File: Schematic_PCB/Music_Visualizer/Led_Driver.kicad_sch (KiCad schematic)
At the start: 92 parts, among them U10 LM3915N-1, U11 LM3915N-1, U12 LM3915N-1, U13 LM3915N-1, U14 LM3915N-1, U15 LM3915N-1, U16 LM3915N-1, U17 NCP161ASN350T1G

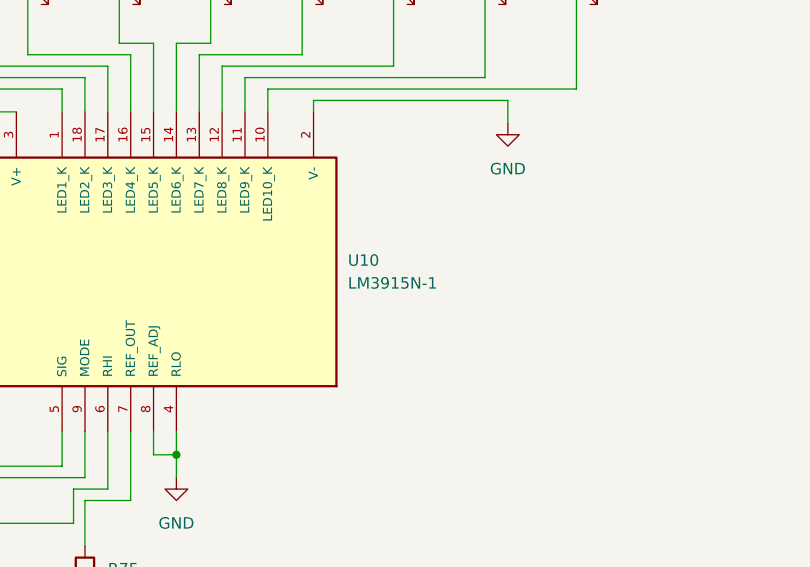
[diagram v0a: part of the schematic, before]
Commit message: Delete unused LED step and fooprint files in the Project library
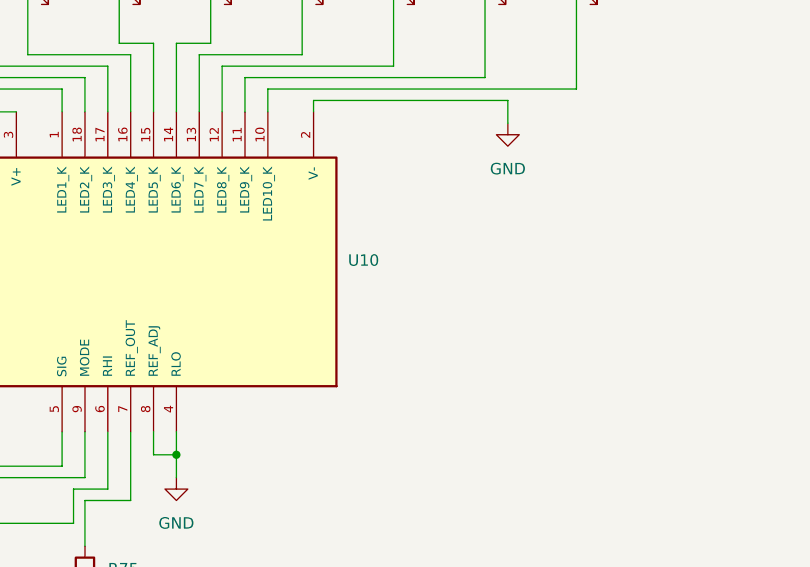
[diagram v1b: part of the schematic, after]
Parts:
- U10: value LM3915N-1 -> (none); footprint Package_DIP:DIP-18_W7.62mm_Socket -> (none)
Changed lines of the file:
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@@
       (effects (font (size 1.27 1.27)) (justify right))
     )
-    (property "Value" "LM3915N-1" (id 1) (at 118.11 90.1699 90)
+    (property "Value" "" (id 1) (at 118.11 90.1699 90)
       (effects (font (size 1.27 1.27)) (justify right))
     )
-    (property "Footprint" "Package_DIP:DIP-18_W7.62mm_Socket" (id 2) (at 96.52 88.9 0)
+    (property "Footprint" "" (id 2) (at 96.52 88.9 0)
       (effects (font (size 1.27 1.27)) (justify left bottom) hide)
     )

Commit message: Rearraged Power circuitry schematic and made the paper size custom: 180W x 250H
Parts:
- RV1: value (none) -> 10k_LED_Brightness_Pot; footprint (none) -> PTV09A_Pot_Vertical:PTV09
- U10: value (none) -> LM3915N-1; footprint (none) -> Package_DIP:DIP-18_W7.62mm_Socket
- U18: value (none) -> NCS333ASQ3T2G; footprint (none) -> Package_TO_SOT_SMD:SOT-353_SC-70-5
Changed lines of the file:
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@@
       (effects (font (size 1.27 1.27)) (justify right))
     )
-    (property "Value" "" (id 1) (at 355.6 212.0899 0)
-      (effects (font (size 1.27 1.27)) (justify right))
-    )
-    (property "Footprint" "" (id 2) (at 358.14 210.82 0)
+    (property "Value" "10k_LED_Brightness_Pot" (id 1) (at 355.6 212.0899 0)
+      (effects (font (size 1.27 1.27)) (justify right))
+    )
+    (property "Footprint" "PTV09A_Pot_Vertical:PTV09" (id 2) (at 358.14 210.82 0)
       (effects (font (size 1.27 1.27)) hide)
     )
@@
     (in_bom yes) (on_board yes) (fields_autoplaced)
     (property "Reference" "U18" (id 0) (at 533.4 211.201 0))
-    (property "Value" "" (id 1) (at 533.4 213.741 0))
-    (property "Footprint" "" (id 2) (at 519.43 215.9 0)
+    (property "Value" "NCS333ASQ3T2G" (id 1) (at 533.4 213.741 0))
+    (property "Footprint" "Package_TO_SOT_SMD:SOT-353_SC-70-5" (id 2) (at 519.43 215.9 0)
       (effects (font (size 1.27 1.27)) (justify left) hide)
     )
@@
       (effects (font (size 1.27 1.27)) (justify right))
     )
-    (property "Value" "" (id 1) (at 118.11 90.1699 90)
-      (effects (font (size 1.27 1.27)) (justify right))
-    )
-    (property "Footprint" "" (id 2) (at 96.52 88.9 0)
-      (effects (font (size 1.27 1.27)) (justify left bottom) hide)
-    )
+    (property "Value" "LM3915N-1" (id 1) (at 118.11 90.1699 90)
+      (effects (font (size 1.27 1.27)) (justify right))
+    )
+    (property "Footprint" "Package_DIP:DIP-18_W7.62mm_Socket" (id 2) (at 96.52 88.9 0)
+      (effects (font (size 1.27 1.27)) (justify left bottom) hide)
+    )
